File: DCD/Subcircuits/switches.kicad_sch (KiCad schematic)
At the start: 7 parts

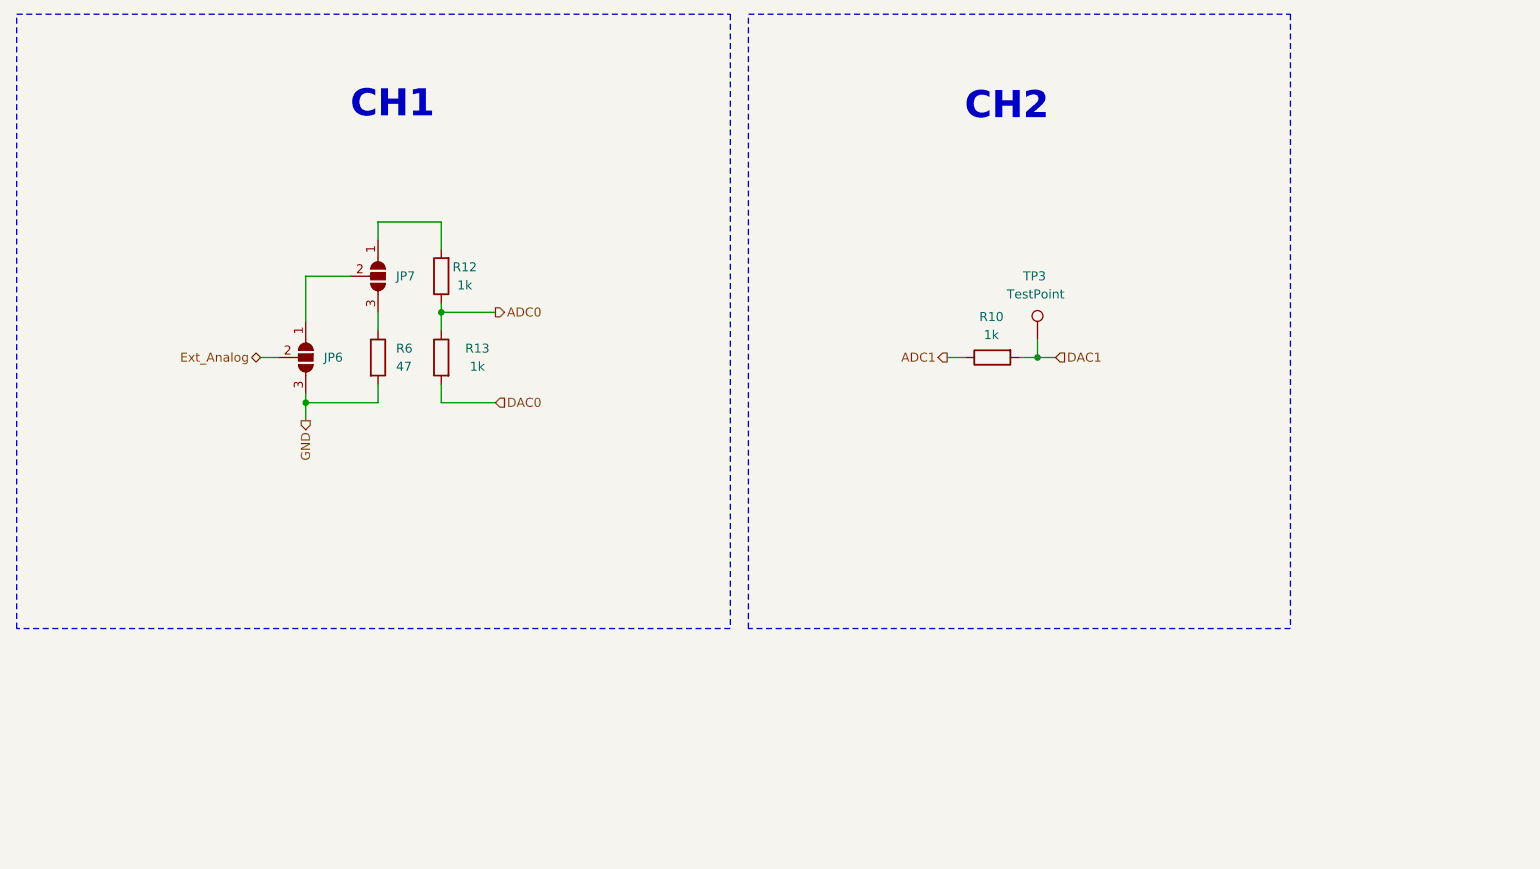
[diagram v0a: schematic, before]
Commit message: Finished the schematics. Fixed the comments that we recieved
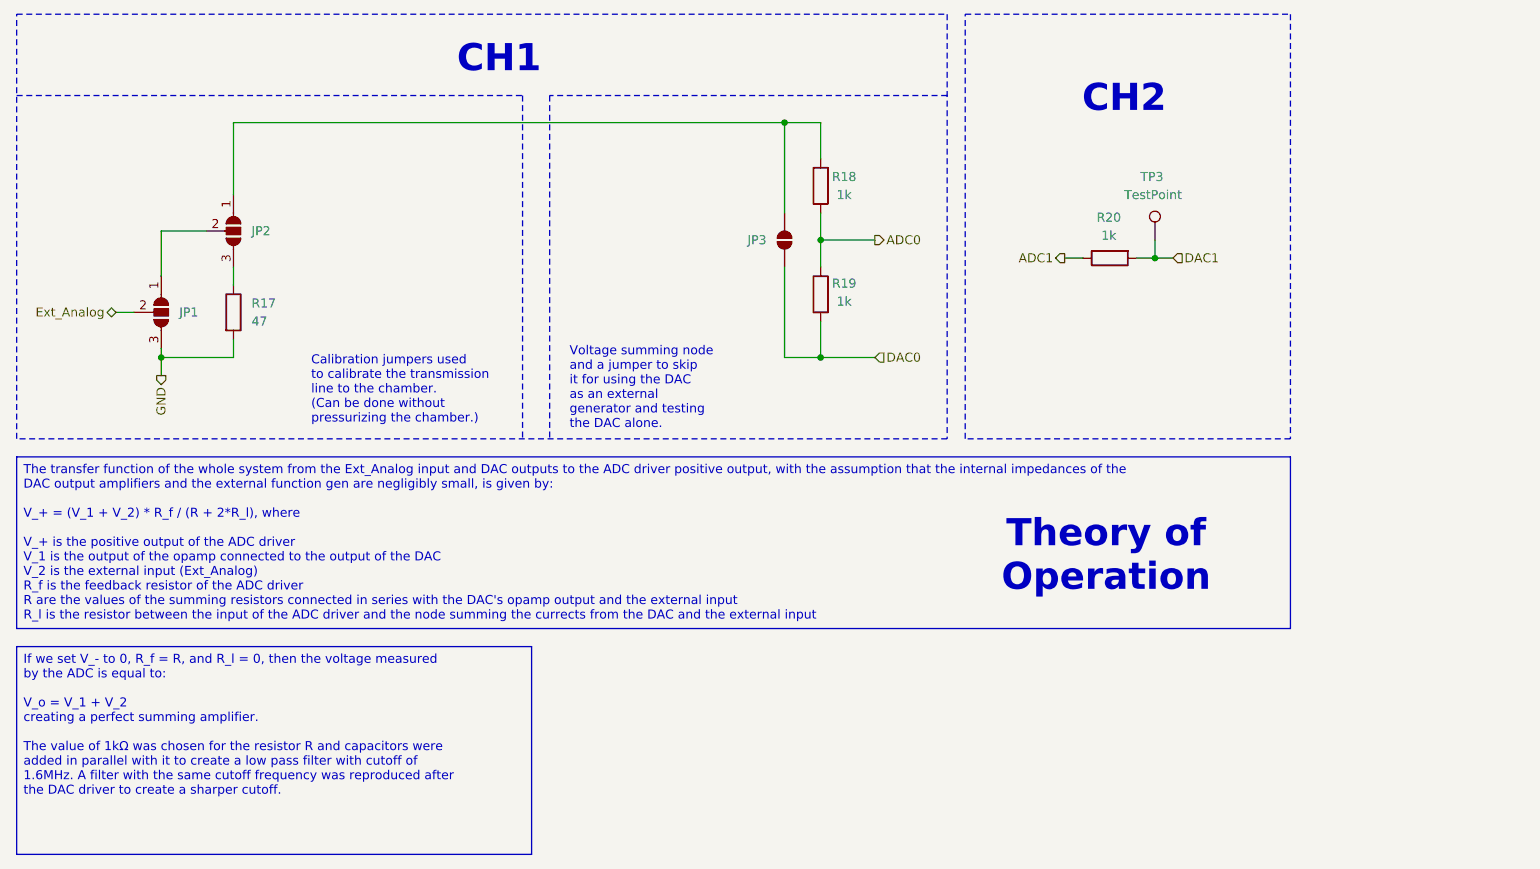
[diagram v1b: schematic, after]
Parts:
- added JP3: SolderJumper_2_Open, Jumper:SolderJumper-2_P1.3mm_Open_RoundedPad1.0x1.5mm, symbol Jumper:SolderJumper_2_Open
- renumbered JP6 to JP1, JP7 to JP2, R6 to R17, R12 to R18, R13 to R19, R10 to R20
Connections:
- net DAC0: now also JP3.1 (A)
- net at JP2.1 (A), R18.2: now also JP3.2 (B)
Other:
- note added: "Calibration jumpers used to calibrate the transmission line to the chamber. (Can be done without pressurizing the chamber.)"
- note added: "Theory of Operation"
- note added: "Voltage summing node and a jumper to skip it for using the DAC as an external generator and testing the DAC alone."
- moved on the sheet: JP1, JP2, R17, R18, R19, R20, TP3
